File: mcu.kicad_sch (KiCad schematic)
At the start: 47 parts, among them U1 STM32U5G9ZJTxQ, Y1 NX2016SA-16MHZ-EXS00A-CS07826, Y2 NX2012SA-32.768K-STD-MUB-1

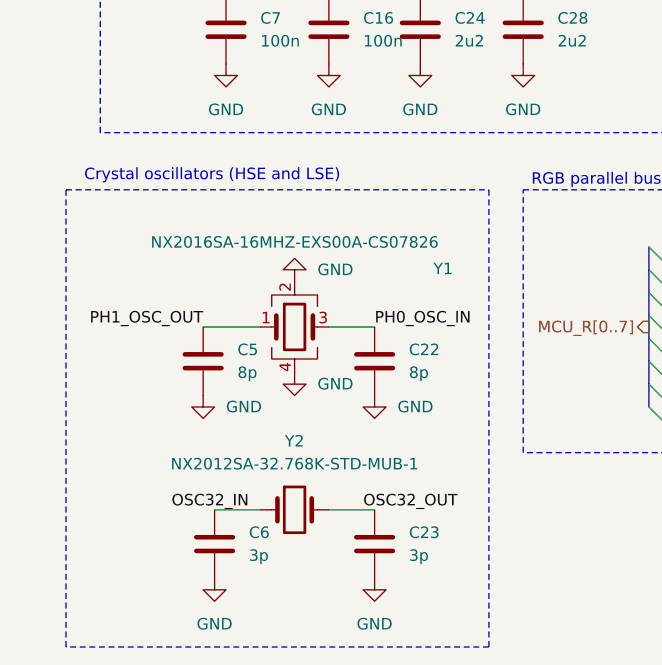
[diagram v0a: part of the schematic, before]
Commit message: End of BOM
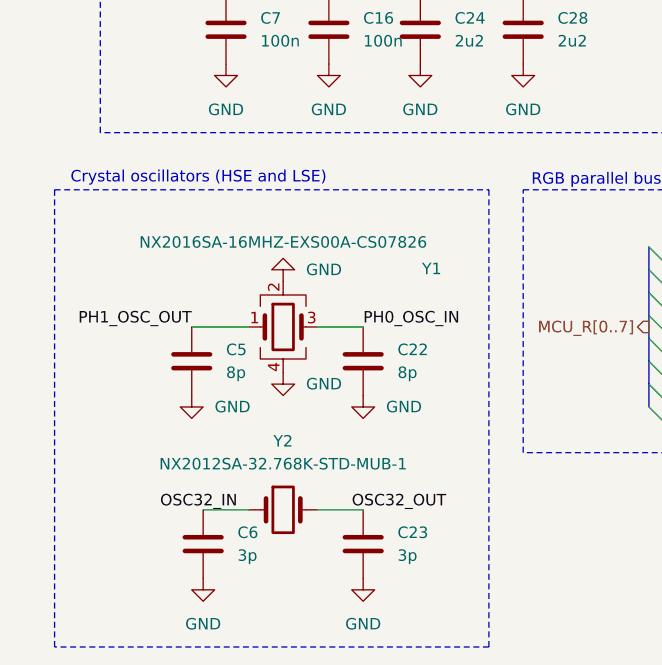
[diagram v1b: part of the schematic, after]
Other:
- moved on the sheet: C22, C23, C5, C6, Y1, Y2
